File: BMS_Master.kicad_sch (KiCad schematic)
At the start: 28 parts, among them U1 STM32F103C8Tx, U2 AP2204K-ADJ, U3 AP2204K-ADJ, U4 SN65HVD256D, Y1 32.768k, Y2 8M

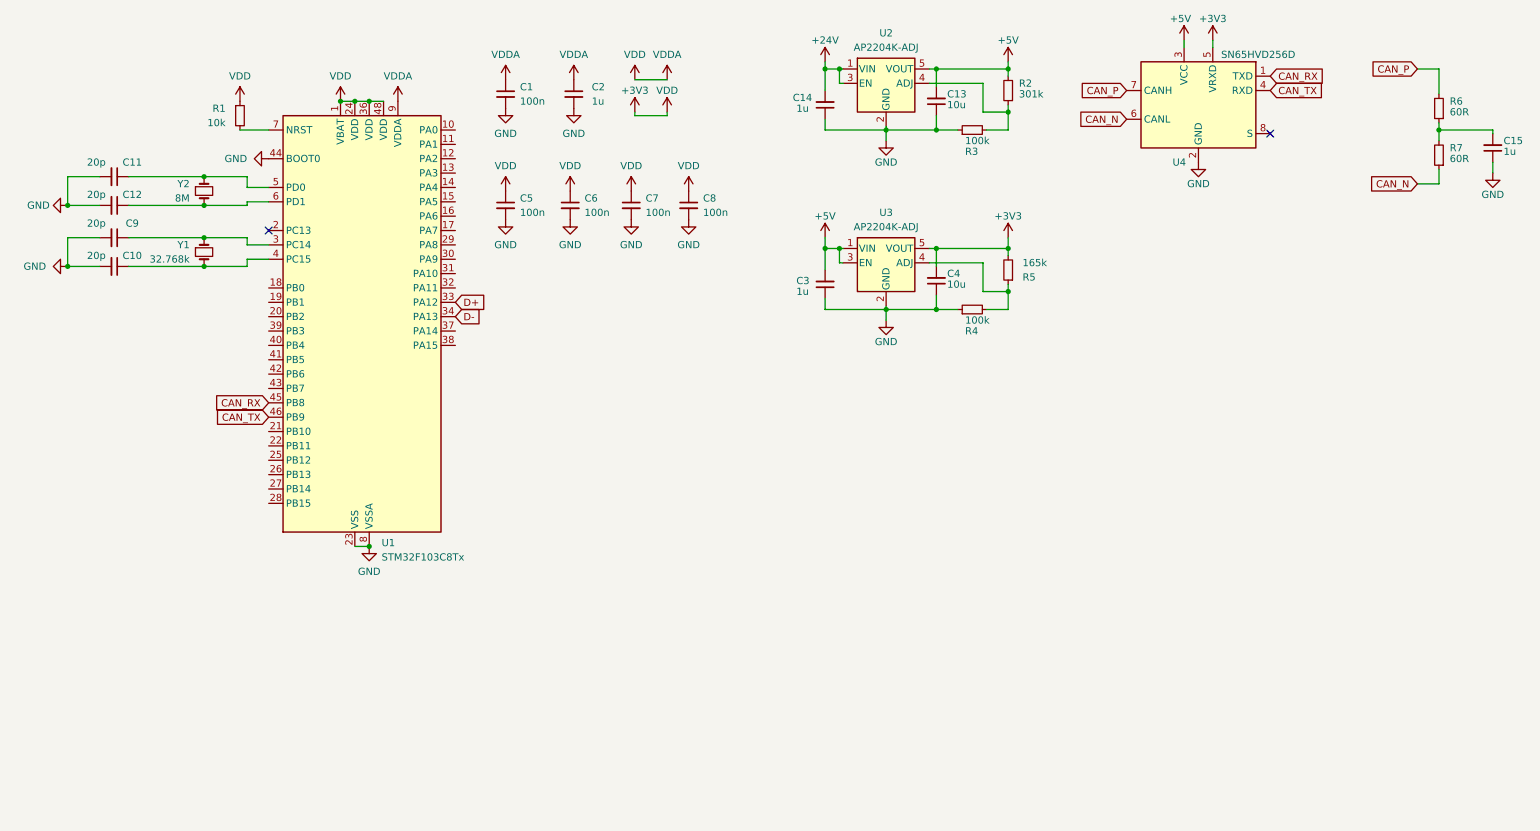
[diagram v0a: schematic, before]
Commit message: Finish schematic (probably)
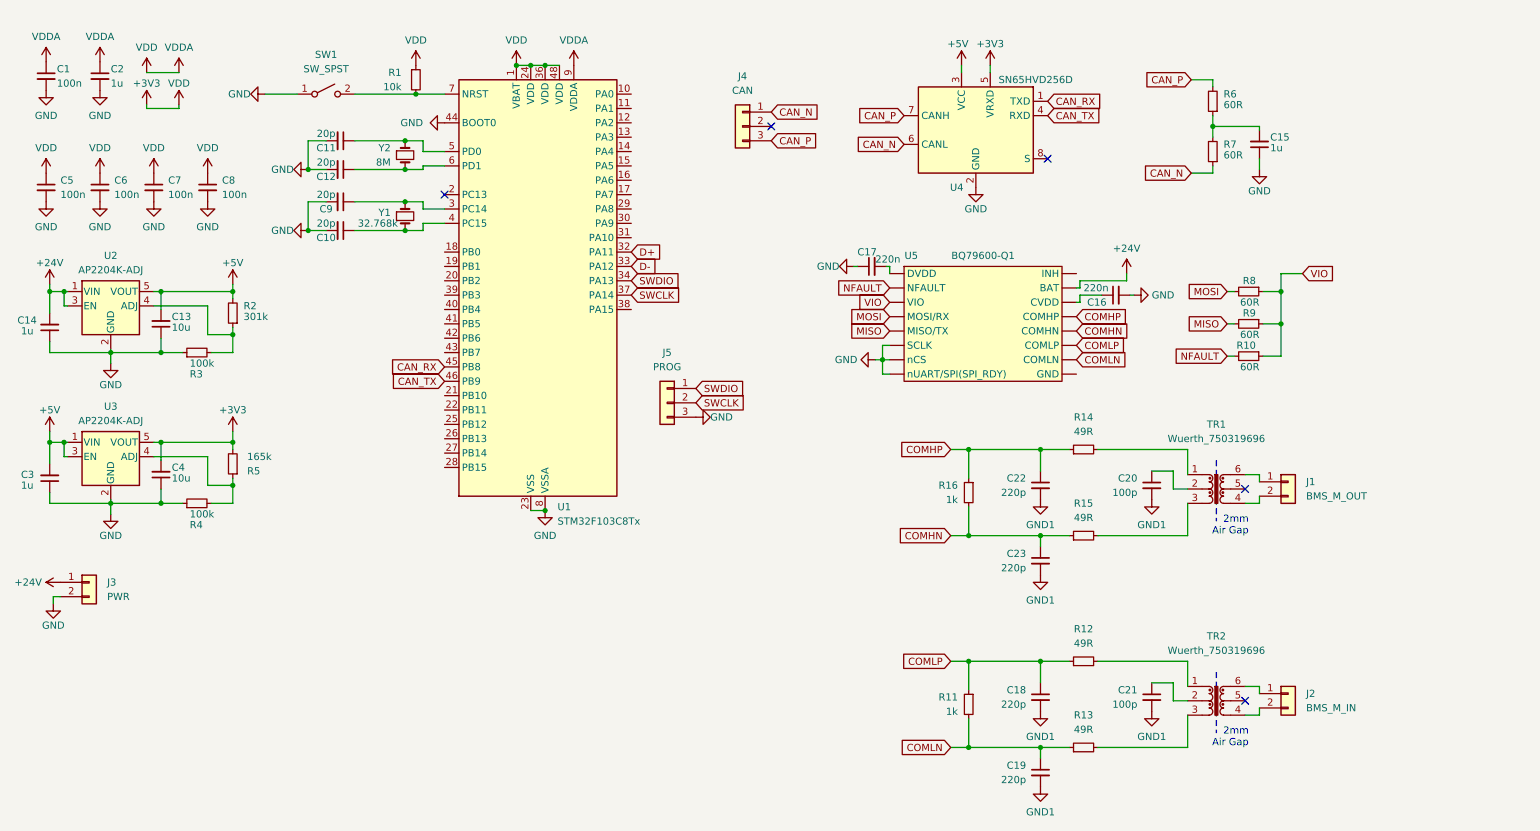
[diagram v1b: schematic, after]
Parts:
- added C16, C17: 220n, Capacitor_SMD:C_0805_2012Metric, symbol Device:C_Small
- added C18, C19, C22, C23: 220p, Capacitor_SMD:C_0603_1608Metric, symbol Device:C_Small
- added C20, C21: 100p, Capacitor_SMD:C_0603_1608Metric, symbol Device:C_Small
- added J1: BMS_M_OUT, Connector_Molex:Molex_Micro-Fit_3.0_43650-0200_1x02_P3.00mm_Horizontal, symbol Connector_Generic:Conn_01x02
- added J2: BMS_M_IN, Connector_Molex:Molex_Micro-Fit_3.0_43650-0200_1x02_P3.00mm_Horizontal, symbol Connector_Generic:Conn_01x02
- added J3: PWR, Connector_JST:JST_XH_S2B-XH-A_1x02_P2.50mm_Horizontal, symbol Connector_Generic:Conn_01x02
- added J4: CAN, Connector_JST:JST_XH_S3B-XH-A_1x03_P2.50mm_Horizontal, symbol Connector_Generic:Conn_01x03
- added J5: PROG, Connector_JST:JST_XH_S3B-XH-A_1x03_P2.50mm_Horizontal, symbol Connector_Generic:Conn_01x03
- added R10, R8, R9: 60R, Resistor_SMD:R_0603_1608Metric, symbol Device:R_Small
- added R11, R16: 1k, Resistor_SMD:R_0603_1608Metric, symbol Device:R_Small
- added R12, R13, R14, R15: 49R, Resistor_SMD:R_0603_1608Metric, symbol Device:R_Small
- added SW1: SW_SPST, symbol Switch:SW_SPST
- added TR1, TR2: Wuerth_750319696, Transformer_SMD:Transformer_Wuerth_750315371, symbol Transformer:Wuerth_750315371
- added U5: BQ79600-Q1, Package_SO:TSSOP-16_4.4x5mm_P0.65mm, symbol Local_Lib:BQ79600-Q1
- C1: footprint Capacitor_SMD:C_0805_2012Metric -> Package_SO:TSSOP-16-1EP_4.4x5mm_P0.65mm
- Y1, Y2: footprint (none) -> Crystal:Crystal_SMD_SeikoEpson_FA238-4Pin_3.2x2.5mm
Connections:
- net +24V: now also J3.1 (Pin_1), U5. (nUART/SPI(SPI_RDY))
- net CAN_N: now also J4.1 (Pin_1)
- net CAN_P: now also J4.3 (Pin_3)
- net D+: now also U1.32 (PA11); no longer U1.33 (PA12)
- net D-: now also U1.33 (PA12); no longer U1.34 (PA13)
- net GND: now also C16.2, C17.1, J3.2 (Pin_2), J5.3 (Pin_3), SW1.1 (A), U5. (nUART/SPI(SPI_RDY))
- net at R1.2, U1.7 (NRST): now also SW1.2 (B)
- net SWCLK: now reaches U1.37 (PA14)
- net SWCLK: now also J5.2 (Pin_2)
- new net: R13.2, TR2.3
- new net: R14.2, TR1.1
- new net: C20.1, TR1.2
- new net: R15.2, TR1.3
- new net: J1.2 (Pin_2), TR1.4
- new net: J1.1 (Pin_1), TR1.6
- new net: C16.1, U5. (nUART/SPI(SPI_RDY))
- new net: C17.2, U5. (nUART/SPI(SPI_RDY))
- new net: C21.1, TR2.2
- new net: J2.1 (Pin_1), TR2.6
- new net: J2.2 (Pin_2), TR2.4
- new net: R12.2, TR2.1
- new net COMHN: C23.1, R15.1, R16.2, U5. (nUART/SPI(SPI_RDY))
- new net COMHP: C22.1, R14.1, R16.1, U5. (nUART/SPI(SPI_RDY))
- new net COMLN: C19.1, R11.2, R13.1, U5. (nUART/SPI(SPI_RDY))
- new net COMLP: C18.1, R11.1, R12.1, U5. (nUART/SPI(SPI_RDY))
- new net GND1: C18.2, C19.2, C20.2, C21.2, C22.2, C23.2
- new net MISO: R9.2, U5. (nUART/SPI(SPI_RDY))
- new net MOSI: R8.2, U5. (nUART/SPI(SPI_RDY))
- new net NFAULT: R10.2, U5. (nUART/SPI(SPI_RDY))
- new net SWDIO: J5.1 (Pin_1), U1.34 (PA13)
- new net VIO: R10.1, R8.1, R9.1, U5. (nUART/SPI(SPI_RDY))
- no-connect marks 2 -> 5
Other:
- note added: "2mm Air Gap"
- moved on the sheet: C1, C10, C11, C12, C13, C14, C15, C2, C3, C4, C5, C6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
